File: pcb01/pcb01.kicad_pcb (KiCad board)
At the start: 2 copper layers, 23 parts, among them SW1 SW_Push, U1 W65C02SxP, U2 HM62256BLP, U3 27C512, U4 PAL20RS10, U5 74LS138, U6 74HCT574, U7 HM62256BLP, U8 R565c52, X1 ACO-xxxMHz, Y1 Crystal

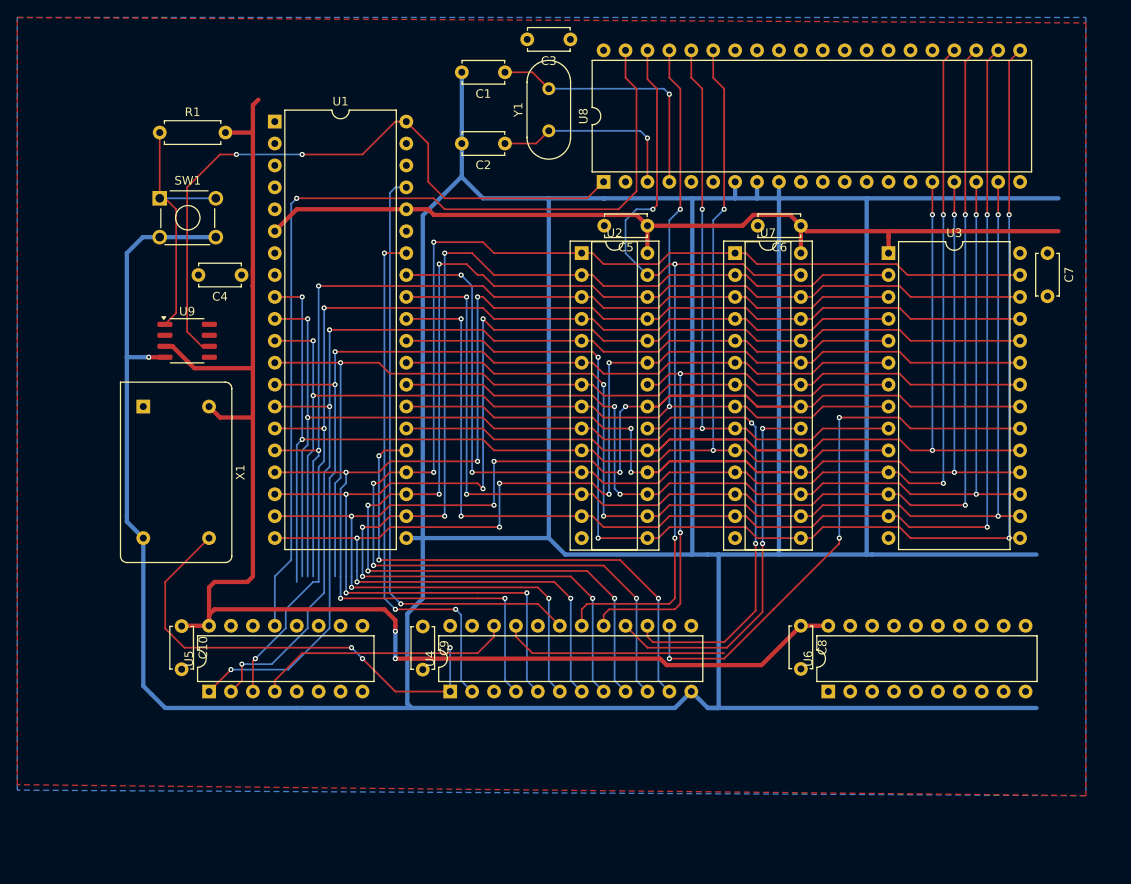
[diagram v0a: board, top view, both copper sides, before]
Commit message: pcb layout should be finished...
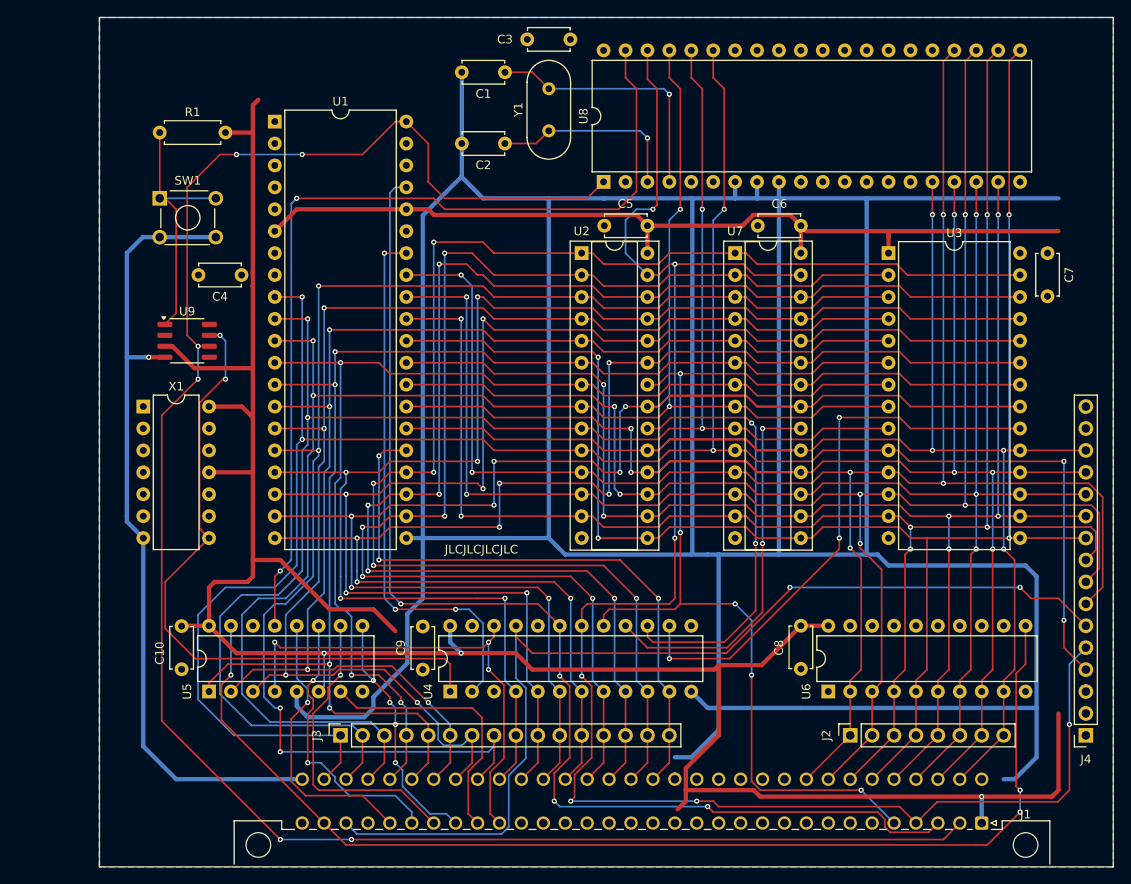
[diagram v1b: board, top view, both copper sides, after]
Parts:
- added J1: DIN41612_02x32_AC, Connector_DIN:DIN41612_C_2x32_Male_Horizontal_THT, F.Cu at (123.8, 113.0)
- added J2: Conn_01x08_Socket, Connector_PinSocket_2.54mm:PinSocket_1x08_P2.54mm_Vertical, F.Cu at (108.6, 102.9)
- added J3: Conn_01x16_Socket, Connector_PinSocket_2.54mm:PinSocket_1x16_P2.54mm_Vertical, F.Cu at (49.5, 102.9)
- added J4: Conn_01x16_Socket, Connector_PinSocket_2.54mm:PinSocket_1x16_P2.54mm_Vertical, F.Cu at (135.9, 102.9)
- X1: footprint Oscillator:Oscillator_DIP-14 -> Package_DIP:DIP-14_W7.62mm
- turned X1 to 0 degrees
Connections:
- U1 pad 25: VCC -> /A15
- U4 pad 11: VCC -> /A15
- U5 pad 10: unconnected-(U5-O5-Pad10) -> /~{IOEN_05}
- U5 pad 11: unconnected-(U5-O4-Pad11) -> /~{IOEN_04}
- U5 pad 12: unconnected-(U5-O3-Pad12) -> /~{IOEN_03}
- U5 pad 7: unconnected-(U5-O7-Pad7) -> /~{IOEN_07}
- U5 pad 9: unconnected-(U5-O6-Pad9) -> /~{IOEN_06}
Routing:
- net /~{RES}: track 78.5 -> 222.8 mm, vias 2 -> 6
- net /~{IOEN_00_GPIO0}: track 0.00 -> 133.8 mm, vias 0 -> 3
- net /~{QWE_RAM}: track 101.0 -> 200.5 mm, vias 3 -> 7
- net /A0: track 154.4 -> 246.3 mm, vias 4 -> 6
- net /DISP_EN: track 26.2 -> 117.6 mm, vias 0 -> 2
- net /A15: track 0.00 -> 72.0 mm, vias 0 -> 3
- net /D0: track 137.7 -> 208.7 mm, vias 4 -> 6
- net /SYS_CLK: track 69.8 -> 138.2 mm, vias 1 -> 4
- net /D1: track 143.5 -> 204.6 mm, vias 4 -> 6
- net /A7: track 107.7 -> 164.4 mm, vias 2 -> 4
- net /D7: track 124.2 -> 173.1 mm, vias 2 -> 4
- net /D2: track 148.6 -> 197.2 mm, vias 4 -> 6
- net /~{QOE}: track 82.6 -> 128.9 mm, vias 2 -> 5
- net /D6: track 131.8 -> 177.7 mm, vias 4 -> 6
- net /A1: track 148.2 -> 192.6 mm
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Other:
- board outline added: 117.5 x 98.4 mm
- board text added: "JLCJLCJLCJLC"
